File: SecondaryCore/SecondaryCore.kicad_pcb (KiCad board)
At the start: 2 copper layers, 88.9 x 35.6 mm, 7 parts, among them J1 Screw_Terminal_01x02, J2 Screw_Terminal_01x02

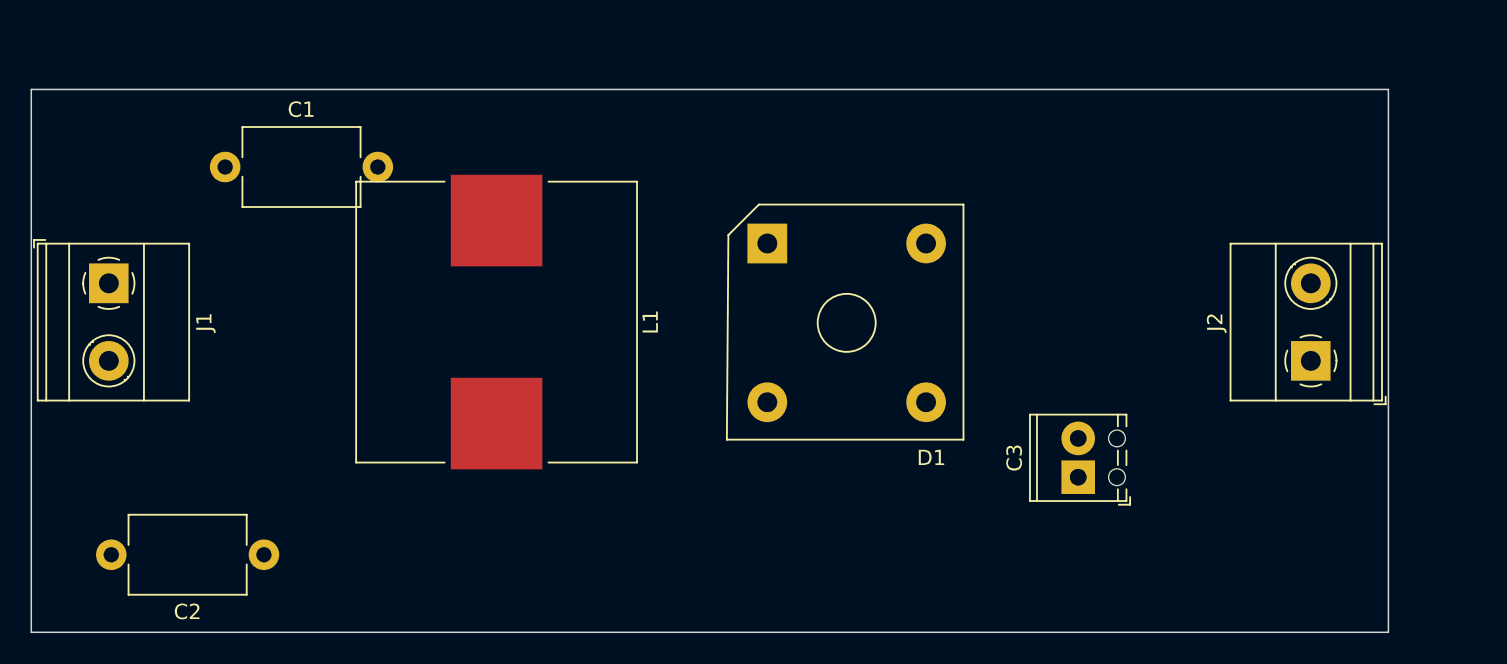
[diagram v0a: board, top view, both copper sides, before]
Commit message: latest route pcb
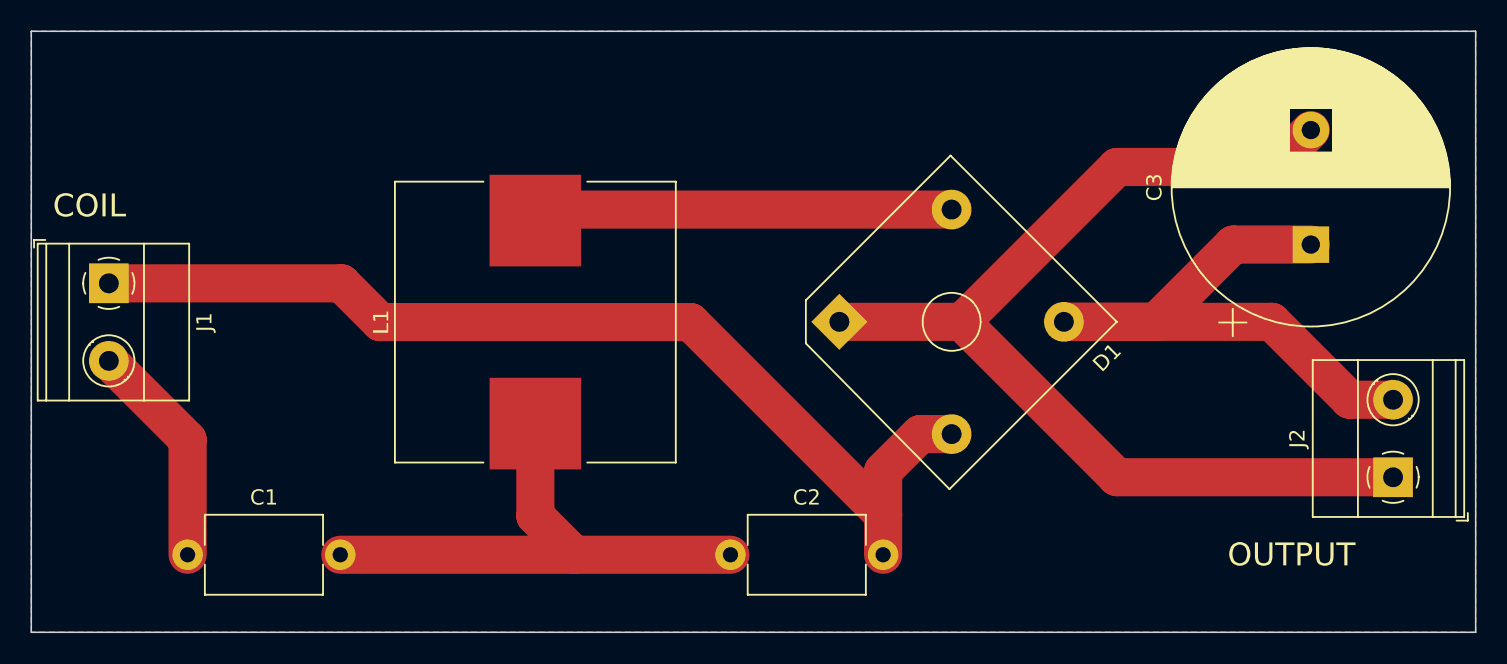
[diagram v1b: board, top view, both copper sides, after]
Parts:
- C3: footprint TerminalBlock_Phoenix:TerminalBlock_Phoenix_MPT-0,5-2-2.54_1x02_P2.54mm_Horizontal -> Capacitor_THT:CP_Radial_D18.0mm_P7.50mm
- moved C2 30.6 mm to (139.8, 106.7), turned to 0 degrees
- moved C1 25.5 mm to (104.2, 106.7)
- moved C3 21.6 mm to (177.8, 86.4)
- moved J2 9.33 mm to (183.2, 101.6)
- moved D1 6.97 mm to (146.9, 91.4), turned to 45 degrees
- moved L1 2.54 mm to (127.0, 91.4), turned to 90 degrees
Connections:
- D1 pad 1: Net-(C3-Pad1) -> Net-(C3-Pad2)
- D1 pad 3: Net-(C3-Pad2) -> Net-(C3-Pad1)
- J2 pad 1: Net-(C3-Pad1) -> Net-(C3-Pad2)
- J2 pad 2: Net-(C3-Pad2) -> Net-(C3-Pad1)
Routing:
- net Net-(C3-Pad2): track 0.00 -> 76.6 mm
- net Net-(C2-Pad2): track 0.00 -> 68.0 mm
- net Net-(C3-Pad1): track 0.00 -> 42.0 mm
- net Net-(C1-Pad2): track 0.00 -> 35.2 mm
- net Net-(D1-Pad4): track 0.00 -> 27.6 mm
- net Net-(C1-Pad1): track 0.00 -> 14.8 mm
- added copper zone on B.Cu, net (none)
- added copper zone on F.Cu, net (none)
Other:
- board size 88.9 x 35.6 mm -> 94.6 x 39.4 mm
- board text added: "COIL"
- board text added: "OUTPUT"
